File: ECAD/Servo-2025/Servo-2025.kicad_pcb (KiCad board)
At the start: 2 copper layers, 25 x 95 mm, 60 parts, among them J1 Conn_02x05_Odd_Even, J10 Conn_01x03, J11 Conn_01x03, J2 Conn_01x02, J3 Conn_01x03, J4 Conn_01x03, J5 Conn_01x03, J6 Conn_01x03, J7 Conn_01x03, J8 Conn_01x03, J9 Conn_01x03

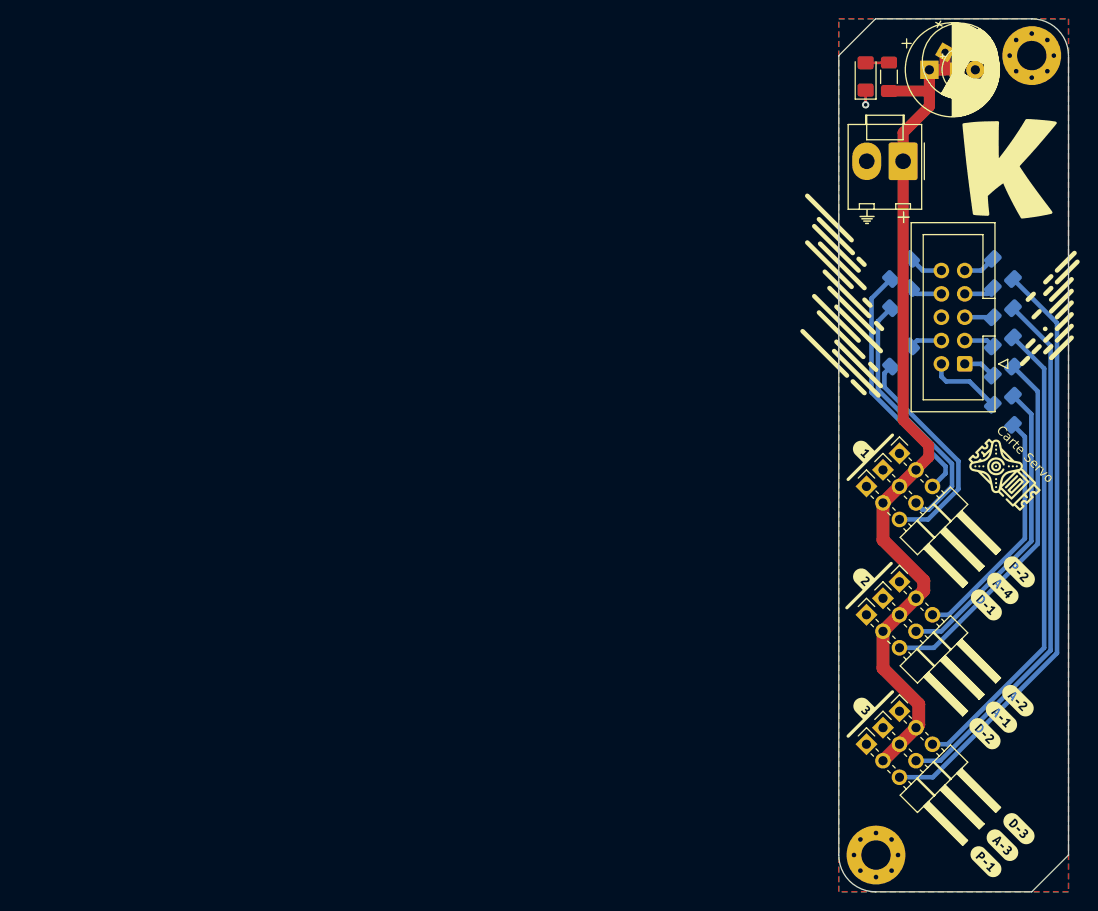
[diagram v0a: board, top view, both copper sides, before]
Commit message: new servo and PCA PBCB
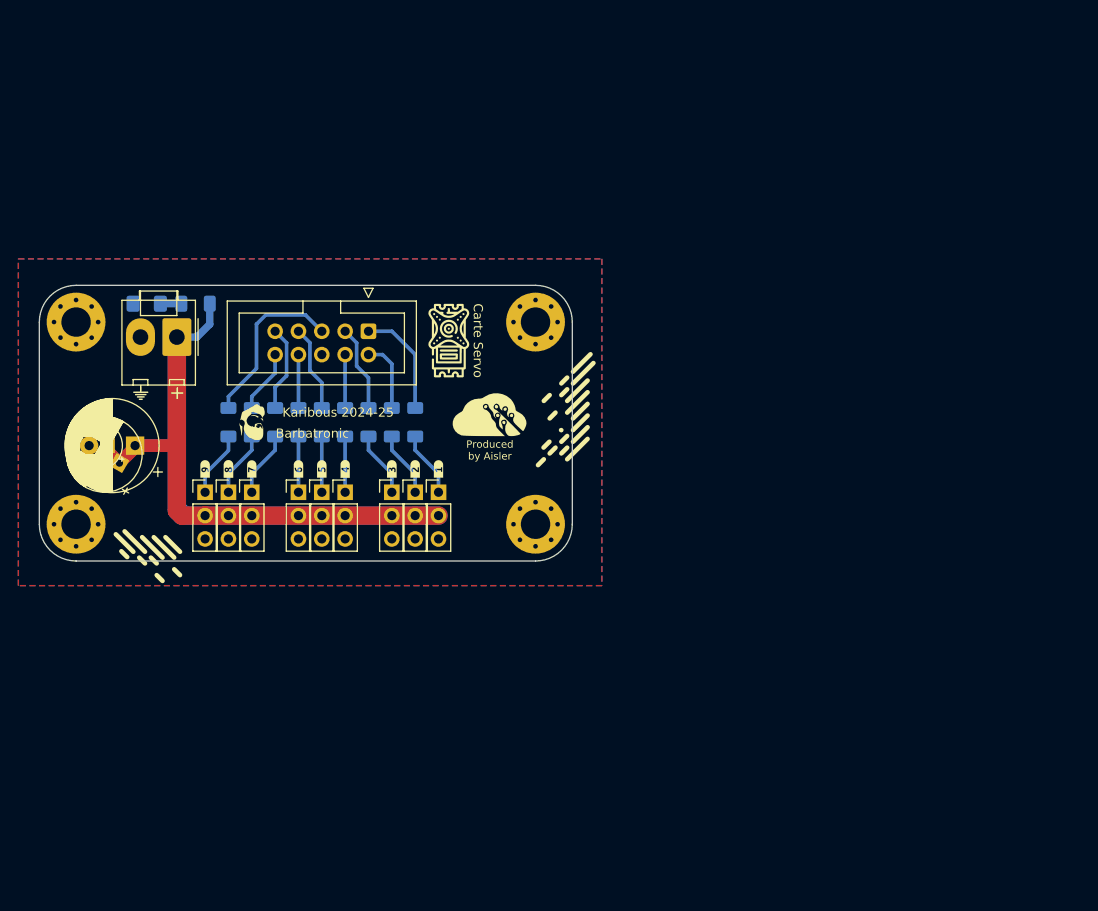
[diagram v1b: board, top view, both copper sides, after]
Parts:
- removed the G*** at (143.9, 77.4)
- removed the G*** at (153.7, 61.6)
- removed kibuzzard-634F18D6 (x2): G***, kibuzzard-634F18D6
- removed kibuzzard-634F18FE (x2): G***, kibuzzard-634F18FE
- removed kibuzzard-634F1907 (x2): G***, kibuzzard-634F1907
- removed kibuzzard-634F19A0 (x2): G***, kibuzzard-634F19A0
- removed kibuzzard-634F19A7 (x2): G***, kibuzzard-634F19A7
- removed kibuzzard-634F19AD (x2): G***, kibuzzard-634F19AD
- removed kibuzzard-634F19FE (x2): G***, kibuzzard-634F19FE
- removed kibuzzard-634F1A03 (x2): G***, kibuzzard-634F1A03
- removed kibuzzard-634F1A09 (x2): G***, kibuzzard-634F1A09
- removed kibuzzard-634F1B38: G***, kibuzzard-634F1B38
- removed kibuzzard-634F1B56: G***, kibuzzard-634F1B56
- removed kibuzzard-634F1B5B: G***, kibuzzard-634F1B5B
- removed kibuzzard-634F1BA4: G***, kibuzzard-634F1BA4
- removed kibuzzard-634F1BAB: G***, kibuzzard-634F1BAB
- removed kibuzzard-634F1BB2: G***, kibuzzard-634F1BB2
- added G***: LOGO, LOGO, F.Cu at (97.0, 88.1)
- added G***: LOGO, LOGO, B.Cu at (105.0, 97.0)
- added G***: LOGO, LOGO, B.Cu at (49.0, 97.0)
- added H3: MountingHole_Pad, MountingHole:MountingHole_3.2mm_M3_Pad_Via, F.Cu at (52.0, 78.0)
- added H4: MountingHole_Pad, MountingHole:MountingHole_3.2mm_M3_Pad_Via, F.Cu at (52.0, 100.0)
- added kibuzzard-679519F0: G***, kibuzzard-679519F0, F.Cu at (91.4, 94.0)
- added kibuzzard-67951A07: G***, kibuzzard-67951A07, F.Cu at (88.9, 94.0)
- added kibuzzard-67951A0B: G***, kibuzzard-67951A0B, F.Cu at (86.4, 94.0)
- added kibuzzard-67951A10: G***, kibuzzard-67951A10, F.Cu at (81.3, 94.0)
- added kibuzzard-67951A14: G***, kibuzzard-67951A14, F.Cu at (78.7, 94.0)
- added kibuzzard-67951A17: G***, kibuzzard-67951A17, F.Cu at (76.2, 94.0)
- added kibuzzard-67951A1B: G***, kibuzzard-67951A1B, F.Cu at (71.1, 94.0)
- added kibuzzard-67951A1E: G***, kibuzzard-67951A1E, F.Cu at (68.6, 94.0)
- added kibuzzard-67951A22: G***, kibuzzard-67951A22, F.Cu at (66.0, 94.0)
- D1, R1: moved to B.Cu
- G***: moved to F.Cu
- J10, J11, J3, J4, J5, J6, J7, J8, J9: footprint Footprints:PinHeader_3x01_P2.54mm_Horizontal -> Connector_PinHeader_2.54mm:PinHeader_1x03_P2.54mm_Vertical
- moved G*** 110.4 mm to (49.0, 81.0), turned to 135 degrees
- moved G*** 102.9 mm to (53.5, 89.0), turned to 0 degrees
- moved C3 101.1 mm to (55.4, 91.4), turned to 180 degrees
- moved C2 100.4 mm to (56.7, 93.3), turned to 150 degrees
- moved G*** 96.9 mm to (71.1, 88.9), turned to 0 degrees
- moved C1 95.6 mm to (58.4, 91.4), turned to 180 degrees
- moved R9 82.8 mm to (71.1, 88.9), turned to 90 degrees
- moved D1 82.0 mm to (59.7, 76.0), turned to 0 degrees
- moved G*** 81.3 mm to (59.0, 85.7)
- moved G*** 81.3 mm to (59.0, 83.0)
- moved J2 81.3 mm to (63.0, 79.6)
- moved R1 79.4 mm to (65.0, 76.0), turned to 180 degrees
- moved J7 79.3 mm to (66.0, 96.5), turned to 0 degrees
- moved R8 79.2 mm to (73.7, 88.9), turned to 90 degrees
- moved R7 76.8 mm to (76.2, 88.9), turned to 90 degrees
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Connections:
- J1 pad 1: IO_A_1 -> C_Act1-1
- J1 pad 10: IO_P_2 -> C_Act1-8
- J1 pad 2: IO_A_2 -> C_Act1-2
- J1 pad 3: IO_D_2 -> C_Act1-3
- J1 pad 4: IO_D_1 -> C_Act1-4
- J1 pad 5: IO_D_3 -> C_Act1-9
- J1 pad 7: IO_A_3 -> C_Act1-5
- J1 pad 8: IO_A_4 -> C_Act1-6
- J1 pad 9: IO_P_1 -> C_Act1-7
- J10 pad 1: GND -> Net-(J10-Pin_1)
- J10 pad 3: Net-(J10-Pad3) -> GND
- J11 pad 1: GND -> Net-(J11-Pin_1)
- J11 pad 3: Net-(J11-Pad3) -> GND
- J3 pad 1: GND -> Net-(J3-Pin_1)
- J3 pad 3: Net-(J3-Pad3) -> GND
- J4 pad 1: GND -> Net-(J4-Pin_1)
- J4 pad 3: Net-(J4-Pad3) -> GND
- J5 pad 1: GND -> Net-(J5-Pin_1)
- J5 pad 3: Net-(J5-Pad3) -> GND
- J6 pad 1: GND -> Net-(J6-Pin_1)
- J6 pad 3: Net-(J6-Pad3) -> GND
- J7 pad 1: GND -> Net-(J7-Pin_1)
- J7 pad 3: Net-(J7-Pad3) -> GND
- J8 pad 1: GND -> Net-(J8-Pin_1)
- J8 pad 3: Net-(J8-Pad3) -> GND
- J9 pad 1: GND -> Net-(J9-Pin_1)
- J9 pad 3: Net-(J9-Pad3) -> GND
- R10 pad 1: Net-(J11-Pad3) -> Net-(J7-Pin_1)
- R10 pad 2: IO_A_4 -> C_Act1-9
- R2 pad 1: Net-(J3-Pad3) -> Net-(J5-Pin_1)
- R2 pad 2: IO_D_1 -> C_Act1-1
- R3 pad 1: Net-(J4-Pad3) -> Net-(J3-Pin_1)
- R3 pad 2: IO_D_2 -> C_Act1-2
- R4 pad 1: Net-(J5-Pad3) -> Net-(J10-Pin_1)
- R4 pad 2: IO_D_3 -> C_Act1-3
- R5 pad 1: Net-(J7-Pad3) -> Net-(J6-Pin_1)
- R5 pad 2: IO_P_1 -> C_Act1-4
- R6 pad 1: Net-(J8-Pad3) -> Net-(J11-Pin_1)
- R6 pad 2: IO_P_2 -> C_Act1-5
- R7 pad 1: Net-(J6-Pad3) -> Net-(J4-Pin_1)
- R7 pad 2: IO_A_1 -> C_Act1-6
- R8 pad 1: Net-(J9-Pad3) -> Net-(J8-Pin_1)
- R8 pad 2: IO_A_2 -> C_Act1-7
- R9 pad 1: Net-(J10-Pad3) -> Net-(J9-Pin_1)
- R9 pad 2: IO_A_3 -> C_Act1-8
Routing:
- net Net-(J7-Pad3): track 65.4 -> 0.00 mm
- net Net-(J10-Pad3): track 58.6 -> 0.00 mm
- net Net-(J5-Pad3): track 51.7 -> 0.00 mm
- net Net-(J4-Pad3): track 40.2 -> 0.00 mm
- net Net-(J6-Pad3): track 33.3 -> 0.00 mm
- net Net-(J11-Pad3): track 28.6 -> 0.00 mm
- net Net-(J8-Pad3): track 27.4 -> 0.00 mm
- net Net-(J9-Pad3): track 26.4 -> 0.00 mm
- net Net-(J3-Pad3): track 24.8 -> 0.00 mm
- net C_Act1-9: track 0.00 -> 18.7 mm
- net +5VP: track 97.5 -> 111.0 mm
- net C_Act1-1: track 0.00 -> 11.9 mm
- net C_Act1-5: track 0.00 -> 9.40 mm
- net C_Act1-3: track 0.00 -> 9.40 mm
- net C_Act1-7: track 0.00 -> 9.39 mm
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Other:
- board size 25 x 95 mm -> 58 x 30 mm
- board text added: "Karibous 2024-25"
- board text added: "Produced by Aisler"
- board text removed: "Karibous 2022-23"
